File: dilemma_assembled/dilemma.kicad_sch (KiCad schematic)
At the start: 102 parts, among them J1 USB_C_Receptacle_USB2.0, J102 NA_serial, J105 NA_Conn_01x04_Female, J113 Cirque, J2 NA_Conn_01x03_Female, J5 Conn_01x02, SW1 SW_Push, SW101 NA_SW_Push, SW102 NA_SW_Push, SW103 NA_SW_Push, SW104 NA_SW_Push, SW105 NA_SW_Push, SW106 NA_SW_Push, SW107 NA_SW_Push, SW108 NA_SW_Push, SW109 NA_SW_Push, SW110 NA_SW_SPST, SW112 NA_SW_Push, SW113 NA_SW_Push, SW114 NA_SW_Push, SW115 NA_SW_Push, SW116 NA_SW_Push, SW117 NA_SW_Push, SW118 NA_SW_Push, SW119 NA_SW_Push, SW2 SW_Push, SW3001 NA_SW_Push, SW3002 NA_RotaryEncoder_Switch, U1 RP2040, U2 GD25Q80CEIGR, U3 XC6210B332MR-G, U4 USBLC6-2P6, Y1 Crystal_GND24

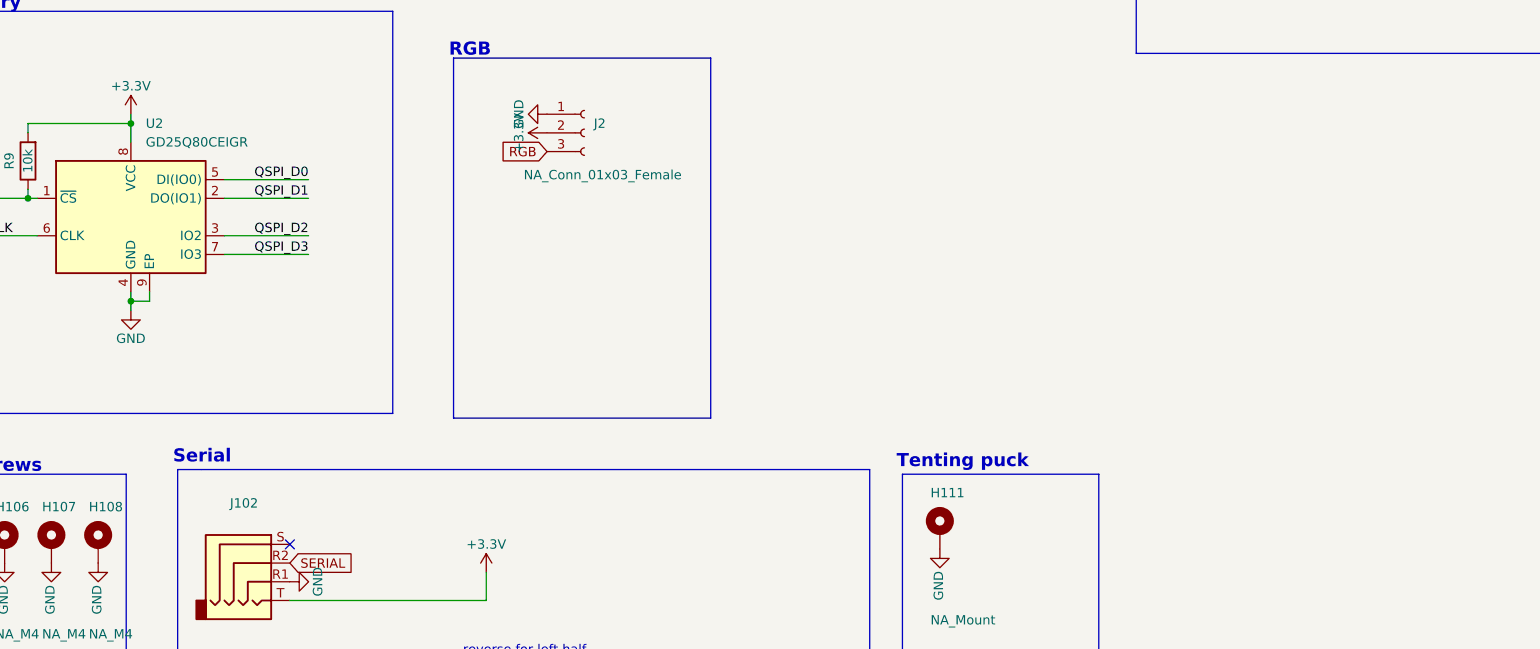
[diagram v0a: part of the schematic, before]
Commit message: change flash memory
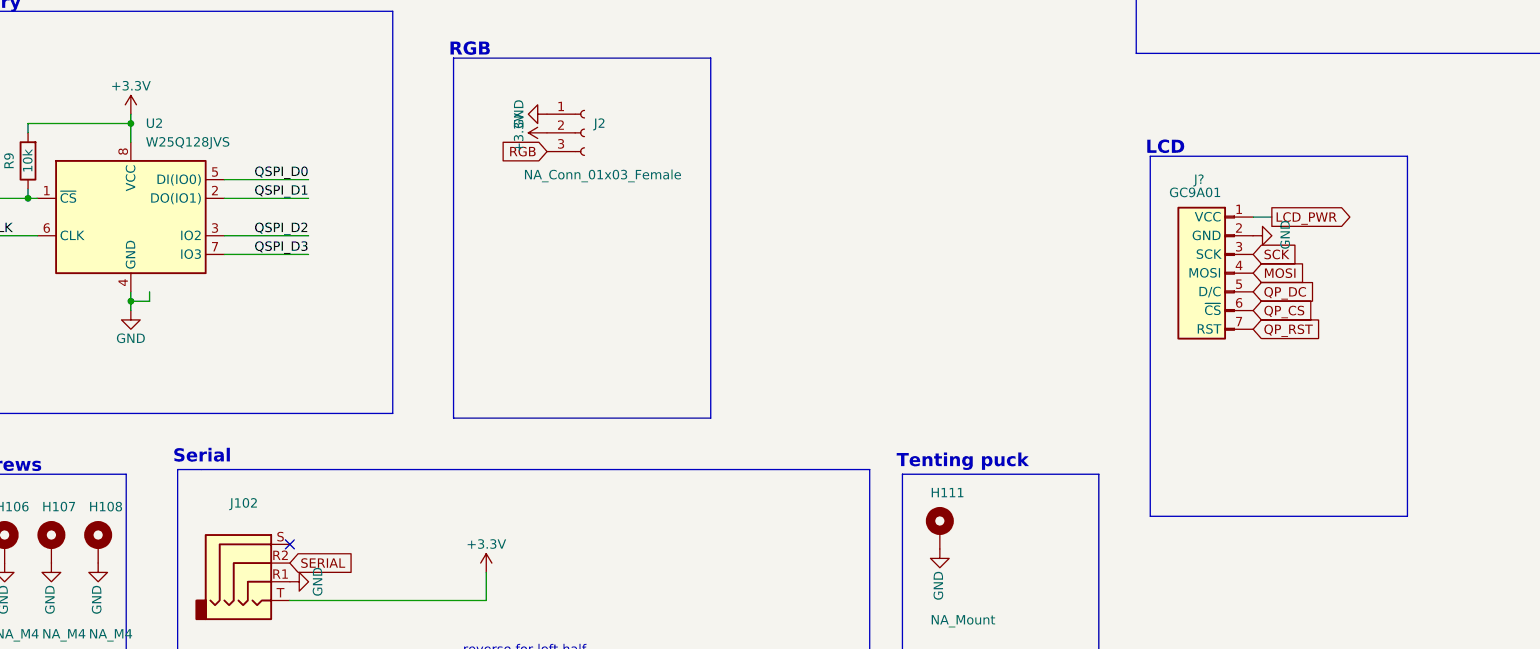
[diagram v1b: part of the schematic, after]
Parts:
- removed U2: GD25Q80CEIGR, 0xLib_Package_DFN_QFN:USON-8-1EP_3x2mm_P0.5mm_EP0.25x1.65mm, symbol Memory_Flash:W25Q32JVZP
- added J?: GC9A01, prettylib:GC9A01-biggers hole, symbol kbd:IPS_LCD__gc9a01_240X240
- added U2: W25Q128JVS, drawings:W25Q128JVPIQ, symbol Memory_Flash:W25Q128JVS
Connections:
- net +3V3: now also U2.8 (VCC)
- net GND: now also J?.2 (GND), U2.4 (GND)
- net MOSI: now also J?.4 (MOSI)
- net QSPI_D0: now also U2.5 (DI(IO0))
- net QSPI_D1: now also U2.2 (DO(IO1))
- net QSPI_D2: now also U2.3 (IO2)
- net QSPI_D3: now also U2.7 (IO3)
- net QSPI_SCLK: now also U2.6 (CLK)
- net QSPI_~{CS}: now also U2.1 (~{CS})
- new net LCD_PWR: J?.1 (VCC)
- new net QP_CS: J?.6 (~{CS})
- new net QP_DC: J?.5 (D/C)
- new net QP_RST: J?.7 (RST)
- new net SCK: J?.3 (SCK)
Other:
- note added: "LCD"
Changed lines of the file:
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@@
     (stroke (width 0) (type default) (color 0 0 0 0))
   )
+  (polyline (pts (xy 417.195 123.825) (xy 417.195 172.72))
+    (stroke (width 0) (type default) (color 0 0 0 0))
+  )
   (wire (pts (xy 71.12 226.06) (xy 97.79 226.06))
     (stroke (width 0) (type default) (color 0 0 0 0))
@@
     (stroke (width 0) (type default) (color 0 0 0 0))
   )
+  (wire (pts (xy 396.24 132.08) (xy 398.78 132.08))
+    (stroke (width 0) (type default) (color 0 0 0 0))
+  )
   (wire (pts (xy 64.135 44.45) (xy 64.135 45.085))
     (stroke (width 0) (type default) (color 0 0 0 0))
@@
     (stroke (width 0) (type default) (color 0 0 0 0))
   )
+  (polyline (pts (xy 382.27 123.825) (xy 382.27 172.72))
+    (stroke (width 0) (type default) (color 0 0 0 0))
+  )
   (wire (pts (xy 97.79 88.9) (xy 127 88.9))
     (stroke (width 0) (type default) (color 0 0 0 0))
@@
     (stroke (width 0) (type default) (color 0 0 0 0))
   )
+  (polyline (pts (xy 417.195 172.72) (xy 382.27 172.72))
+    (stroke (width 0) (type default) (color 0 0 0 0))
+  )
   (wire (pts (xy 123.825 120.65) (xy 127 120.65))
     (stroke (width 0) (type default) (color 0 0 0 0))
@@
     (stroke (width 0) (type default) (color 0 0 0 0))
   )
+  (polyline (pts (xy 382.27 123.825) (xy 417.195 123.825))
+    (stroke (width 0) (type default) (color 0 0 0 0))
+  )
   (wire (pts (xy 54.61 113.03) (xy 58.42 113.03))
     (stroke (width 0) (type default) (color 0 0 0 0))
@@
     (effects (font (size 1.778 1.778) (thickness 0.3556) bold) (justify right bottom))
   )
+  (text "LCD" (at 381.635 123.825 0)
+    (effects (font (size 1.778 1.778) (thickness 0.3556) bold) (justify left bottom))
+  )
   (text "Cirque FPC connector" (at 320.04 19.685 0)
     (effects (font (size 1.778 1.778) (thickness 0.3556) bold) (justify left bottom))
@@
     )
   )
+  (global_label "SCK" (shape input) (at 396.24 137.16 0) (fields_autoplaced)
+    (effects (font (size 1.27 1.27)) (justify left))
+    (property "Intersheet References" "${INTERSHEET_REFS}" (id 0) (at 402.4026 137.0806 0)
+      (effects (font (size 1.27 1.27)) (justify left) hide)
+    )
+  )
   (global_label "M_ROW3" (shape input) (at 33.02 226.06 180)
     (effects (font (size 1.27 1.27)) (justify right))
@@
     )
   )
+  (global_label "QP_RST" (shape input) (at 396.24 147.32 0) (fields_autoplaced)
+    (effects (font (size 1.27 1.27)) (justify left))
+    (property "Intersheet References" "${INTERSHEET_REFS}" (id 0) (at 405.6683 147.2406 0)
+      (effects (font (size 1.27 1.27)) (justify left) hide)
+    )
+  )
   (global_label "SDA" (shape input) (at 329.565 35.56 180)
     (effects (font (size 1.27 1.27)) (justify right))
@@
     )
   )
+  (global_label "QP_DC" (shape input) (at 396.24 142.24 0) (fields_autoplaced)
+    (effects (font (size 1.27 1.27)) (justify left))
+    (property "Intersheet References" "${INTERSHEET_REFS}" (id 0) (at 404.7612 142.1606 0)
+      (effects (font (size 1.27 1.27)) (justify left) hide)
+    )
+  )
   (global_label "M_ROW1" (shape input) (at 182.88 127 0)
     (effects (font (size 1.27 1.27)) (justify left))
@@
     )
   )
+  (global_label "LCD_PWR" (shape output) (at 398.78 132.08 0) (fields_autoplaced)
+    (effects (font (size 1.27 1.27)) (justify left))
+    (property "Intersheet References" "${INTERSHEET_REFS}" (id 0) (at 129.54 -330.2 0)
+      (effects (font (size 1.27 1.27)) hide)
+    )
+  )
   (global_label "RGB" (shape input) (at 182.88 58.42 0)
     (effects (font (size 1.27 1.27)) (justify left))
@@
     )
   )
+  (global_label "QP_CS" (shape input) (at 396.24 144.78 0) (fields_autoplaced)
+    (effects (font (size 1.27 1.27)) (justify left))
+    (property "Intersheet References" "${INTERSHEET_REFS}" (id 0) (at 404.7007 144.7006 0)
+      (effects (font (size 1.27 1.27)) (justify left) hide)
+    )
+  )
+  (global_label "MOSI" (shape input) (at 396.24 139.7 0) (fields_autoplaced)
+    (effects (font (size 1.27 1.27)) (justify left))
+    (property "Intersheet References" "${INTERSHEET_REFS}" (id 0) (at 403.2493 139.6206 0)
+      (effects (font (size 1.27 1.27)) (justify left) hide)
+    )
+  )
   (global_label "NCS" (shape input) (at 342.265 53.34 180)
     (effects (font (size 1.27 1.27)) (justify right))
@@
     (pin "2")
   )
-  (symbol (lib_id "Memory_Flash:W25Q32JVZP") (at 243.84 132.08 0) (unit 1)
-    (in_bom yes) (on_board yes) (fields_autoplaced)
-    (property "Reference" "U2" (id 0) (at 245.8594 119.38 0)
-      (effects (font (size 1.27 1.27)) (justify left))
-    )
-    (property "Value" "GD25Q80CEIGR" (id 1) (at 245.8594 121.92 0)
-      (effects (font (size 1.27 1.27)) (justify left))
-    )
-    (property "Footprint" "0xLib_Package_DFN_QFN:USON-8-1EP_3x2mm_P0.5mm_EP0.25x1.65mm" (id 2) (at 243.84 132.08 0)
-      (effects (font (size 1.27 1.27)) hide)
-    )
-    (property "Datasheet" "" (id 3) (at 243.84 132.08 0)
-      (effects (font (size 1.27 1.27)) hide)
-    )
-    (property "LCSC" "C395484" (id 4) (at 243.84 132.08 0)
-      (effects (font (size 1.27 1.27)) hide)
-    )
-    (pin "1")
-    (pin "2")
-    (pin "3")
-    (pin "4")
-    (pin "5")
-    (pin "6")
-    (pin "7")
-    (pin "8")
-    (pin "9")
-  )
   (symbol (lib_id "Device:D_Dual_CommonCathode_AAK") (at 88.9 247.65 90) (unit 1)
     (in_bom yes) (on_board yes) (fields_autoplaced)
@@
     (pin "1")
   )
+  (symbol (lib_id "kbd:IPS_LCD__gc9a01_240X240") (at 392.43 139.7 0) (mirror y) (unit 1)
+    (in_bom no) (on_board yes)
+    (property "Reference" "J?" (id 0) (at 389.636 127 0)
+      (effects (font (size 1.27 1.27)) (justify left))
+    )
+    (property "Value" "GC9A01" (id 1) (at 391.922 128.778 0)
+      (effects (font (size 1.27 1.27)) (justify left))
+    )
+    (property "Footprint" "prettylib:GC9A01-biggers hole" (id 2) (at 391.16 124.46 0)
+      (effects (font (size 1.27 1.27)) hide)
+    )
+    (property "Datasheet" "~" (id 3) (at 391.16 124.46 0)
+      (effects (font (size 1.27 1.27)) hide)
+    )
+    (pin "1")
+    (pin "2")
+    (pin "3")
+    (pin "4")
+    (pin "5")
+    (pin "6")
+    (pin "7")
+  )
   (symbol (lib_id "Device:C") (at 91.44 180.34 0) (unit 1)
     (in_bom yes) (on_board yes)
@@
     (pin "9")
   )
+  (symbol (lib_id "Memory_Flash:W25Q128JVS") (at 243.84 132.08 0) (unit 1)
+    (in_bom yes) (on_board yes) (fields_autoplaced)
+    (property "Reference" "U2" (id 0) (at 245.8594 119.38 0)
+      (effects (font (size 1.27 1.27)) (justify left))
+    )
+    (property "Value" "W25Q128JVS" (id 1) (at 245.8594 121.92 0)
+      (effects (font (size 1.27 1.27)) (justify left))
+    )
+    (property "Footprint" "drawings:W25Q128JVPIQ" (id 2) (at 243.84 132.08 0)
+      (effects (font (size 1.27 1.27)) hide)
+    )
+    (property "Datasheet" "http://www.winbond.com/resource-files/w25q128jv_dtr%20revc%2003272018%20plus.pdf" (id 3) (at 243.84 132.08 0)
+      (effects (font (size 1.27 1.27)) hide)
+    )
+    (pin "1")
+    (pin "2")
+    (pin "3")
+    (pin "4")
+    (pin "5")
+    (pin "6")
+    (pin "7")
+    (pin "8")
+  )
   (symbol (lib_id "Mechanical:MountingHole_Pad") (at 220.345 176.53 0) (unit 1)
     (in_bom yes) (on_board yes)
@@
     (pin "1")
   )
+  (symbol (lib_id "power:GND") (at 396.24 134.62 90) (unit 1)
+    (in_bom yes) (on_board yes)
+    (property "Reference" "#PWR?" (id 0) (at 402.59 134.62 0)
+      (effects (font (size 1.27 1.27)) hide)
+    )
+    (property "Value" "GND" (id 1) (at 400.6342 134.493 0))
+    (property "Footprint" "" (id 2) (at 396.24 134.62 0)
+      (effects (font (size 1.27 1.27)) hide)
+    )
+    (property "Datasheet" "" (id 3) (at 396.24 134.62 0)
+      (effects (font (size 1.27 1.27)) hide)
+    )
+    (pin "1")
+  )
   (symbol (lib_id "Device:C") (at 130.81 180.34 0) (unit 1)
     (in_bom yes) (on_board yes)
@@
       (reference "#PWR0132") (unit 1) (value "+3.3V") (footprint "")
     )
+    (path "/f1f8c5e8-84ec-46cc-976a-c595f2716600"
+      (reference "#PWR?") (unit 1) (value "GND") (footprint "")
+    )
     (path "/4a21e78b-0ab0-4b88-8132-9b174e045719"
       (reference "C1") (unit 1) (value "1µ") (footprint "Capacitor_SMD:C_0603_1608Metric")
@@
       (reference "J113") (unit 1) (value "Cirque") (footprint "local-libraries:FPC-SMD_FPC05012-09200-.5mm")
     )
+    (path "/6e2411cd-fd67-4be2-b1a3-b3e54de4894a"
+      (reference "J?") (unit 1) (value "GC9A01") (footprint "prettylib:GC9A01-biggers hole")
+    )
     (path "/66096f4f-c798-4425-8537-e7adeb21bec3"
       (reference "O101") (unit 1) (value "NA_OLED") (footprint "local-libraries:PinHeader_1x04_P2.54mm_Vertical")
@@
       (reference "U1") (unit 1) (value "RP2040") (footprint "0xLib_Package_DFN_QFN:QFN-56-1EP_7x7mm_P0.4mm_EP3.2x3.2mm")
     )
-    (path "/3b628cb4-77fa-40d4-8aa3-0ae0b973ec32"
-      (reference "U2") (unit 1) (value "GD25Q80CEIGR") (footprint "0xLib_Package_DFN_QFN:USON-8-1EP_3x2mm_P0.5mm_EP0.25x1.65mm")
+    (path "/f05b539d-f3ed-4d87-8562-322d3113dab5"
+      (reference "U2") (unit 1) (value "W25Q128JVS") (footprint "drawings:W25Q128JVPIQ")
     )
     (path "/33208a57-5054-4bad-b85f-35da7b25e7bb"
